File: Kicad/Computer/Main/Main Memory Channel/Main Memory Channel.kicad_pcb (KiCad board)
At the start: 2 copper layers, 18.8 x 53.5 mm, 14 parts, among them IC1 74LVC541APW,118, IC2 74LVC573APW,118, IC3 74LVC138APW-Q100J, IC4 74LVC573APW,118, IC5 AP7365-33WG-7, IC7 74LVC04APW,118, J4 Conn_02x20_Counter_Clockwise

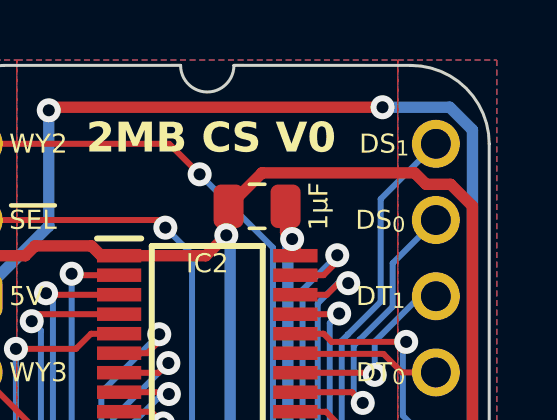
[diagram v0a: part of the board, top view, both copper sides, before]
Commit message: Generated Gerbers for the Mainboard Small and Components.
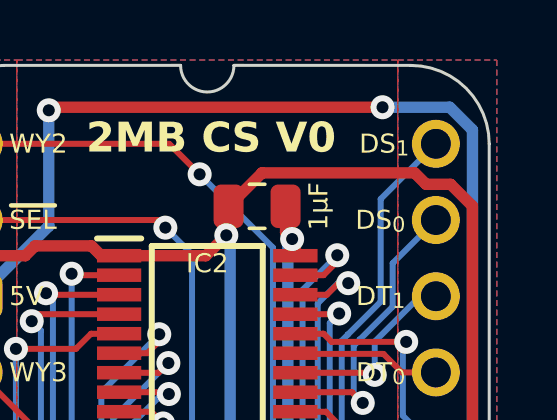
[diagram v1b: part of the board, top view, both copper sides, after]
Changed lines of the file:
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@@
 		(fp_arc
 			(start 14.404267 -2.613733)
-			(mid 16.252448 -1.848183)
+			(mid 16.252451 -1.848184)
 			(end 17.017999 -0.000001)
 			(stroke
